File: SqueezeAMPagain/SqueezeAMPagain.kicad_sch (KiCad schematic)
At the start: 6 parts

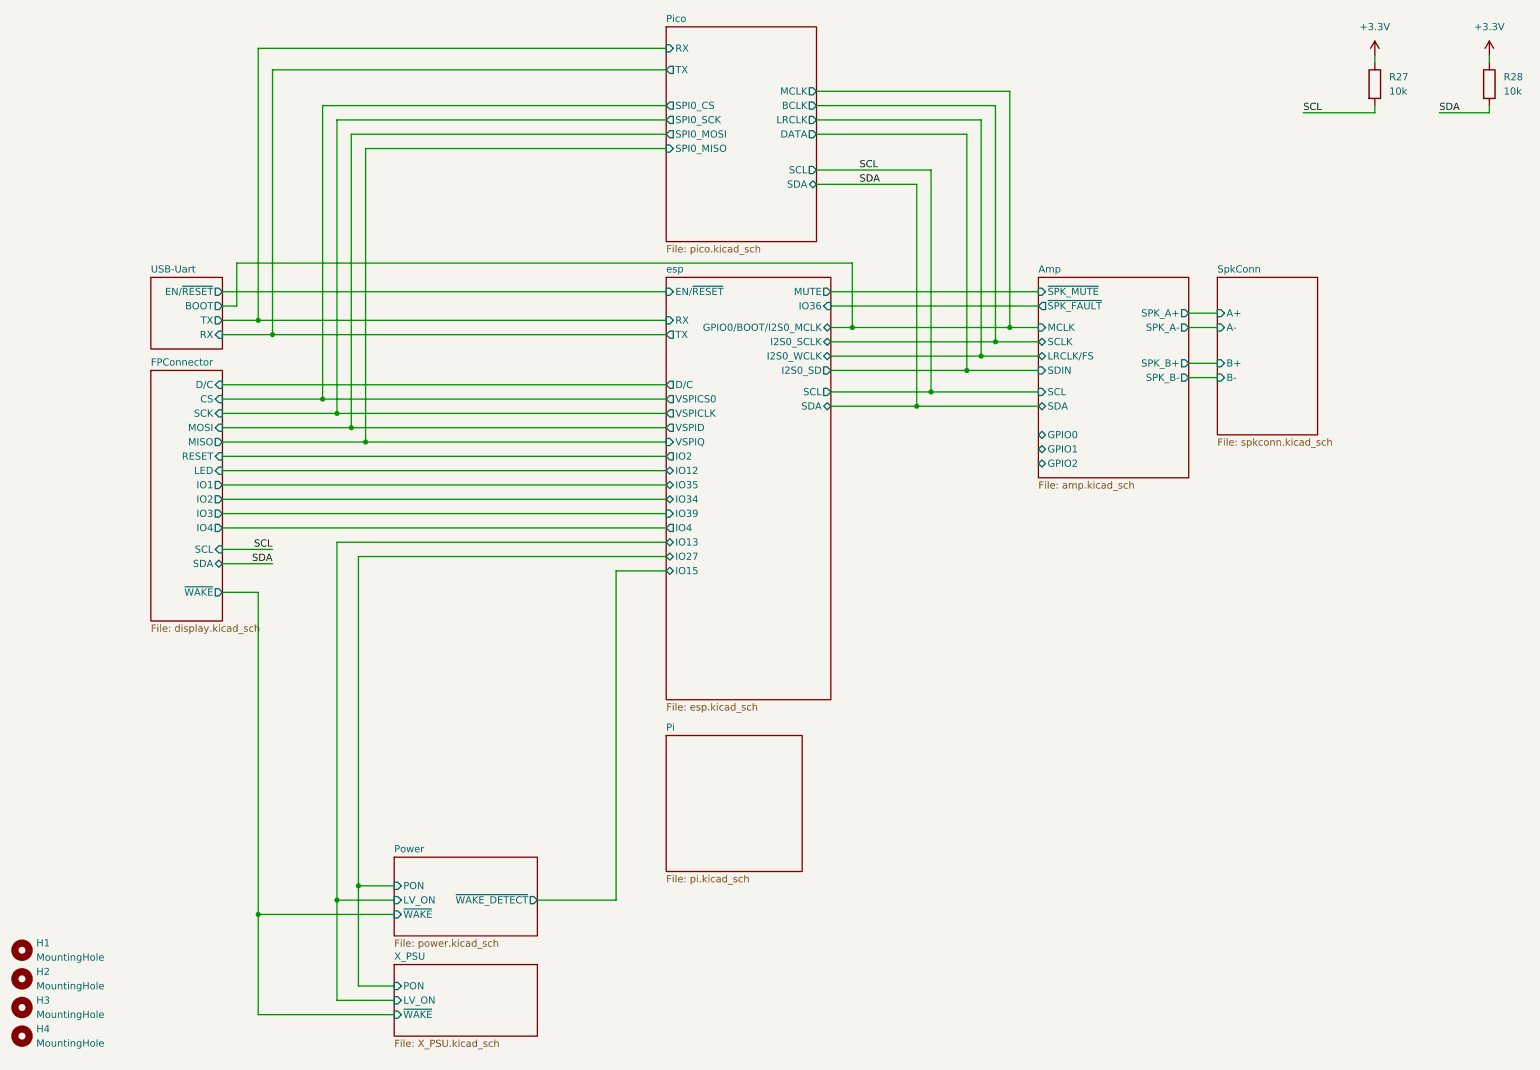
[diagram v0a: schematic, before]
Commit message: Update SqueezeAMPagain.kicad_pcb, SqueezeAMPagain.kicad_prl, SqueezeAMPagain.kicad_pro, and 7 more files
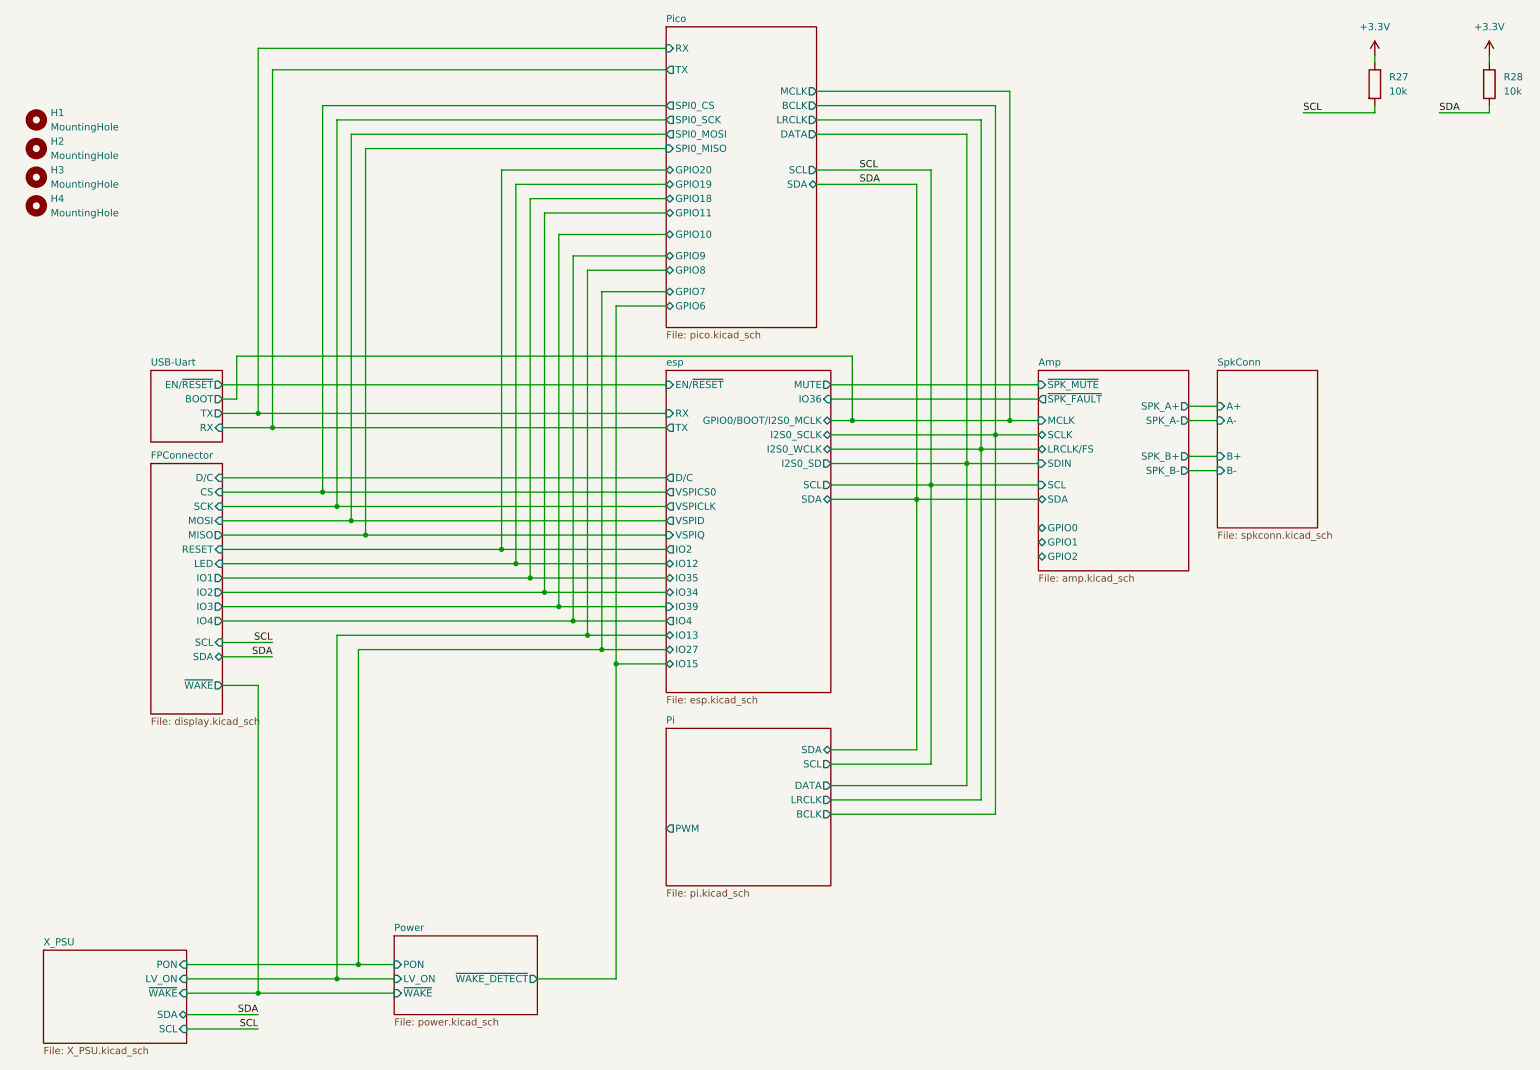
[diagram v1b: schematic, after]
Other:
- sheet Pi ports: added BCLK, DATA, LRCLK, PWM, SCL, SDA; removed none
- sheet Pico ports: added GPIO10, GPIO11, GPIO18, GPIO19, GPIO20, GPIO6, GPIO7, GPIO8, GPIO9; removed none
- sheet X_PSU ports: added SCL, SDA; removed none
- moved on the sheet: H1, H2, H3, H4

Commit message: Update L_Radial_D12.0mm_P5+6+7.00mm_Fastron_11P.kicad_mod, SqueezeAMPagain.kicad_pcb, SqueezeAMPagain.kicad_prl, and 5 more files
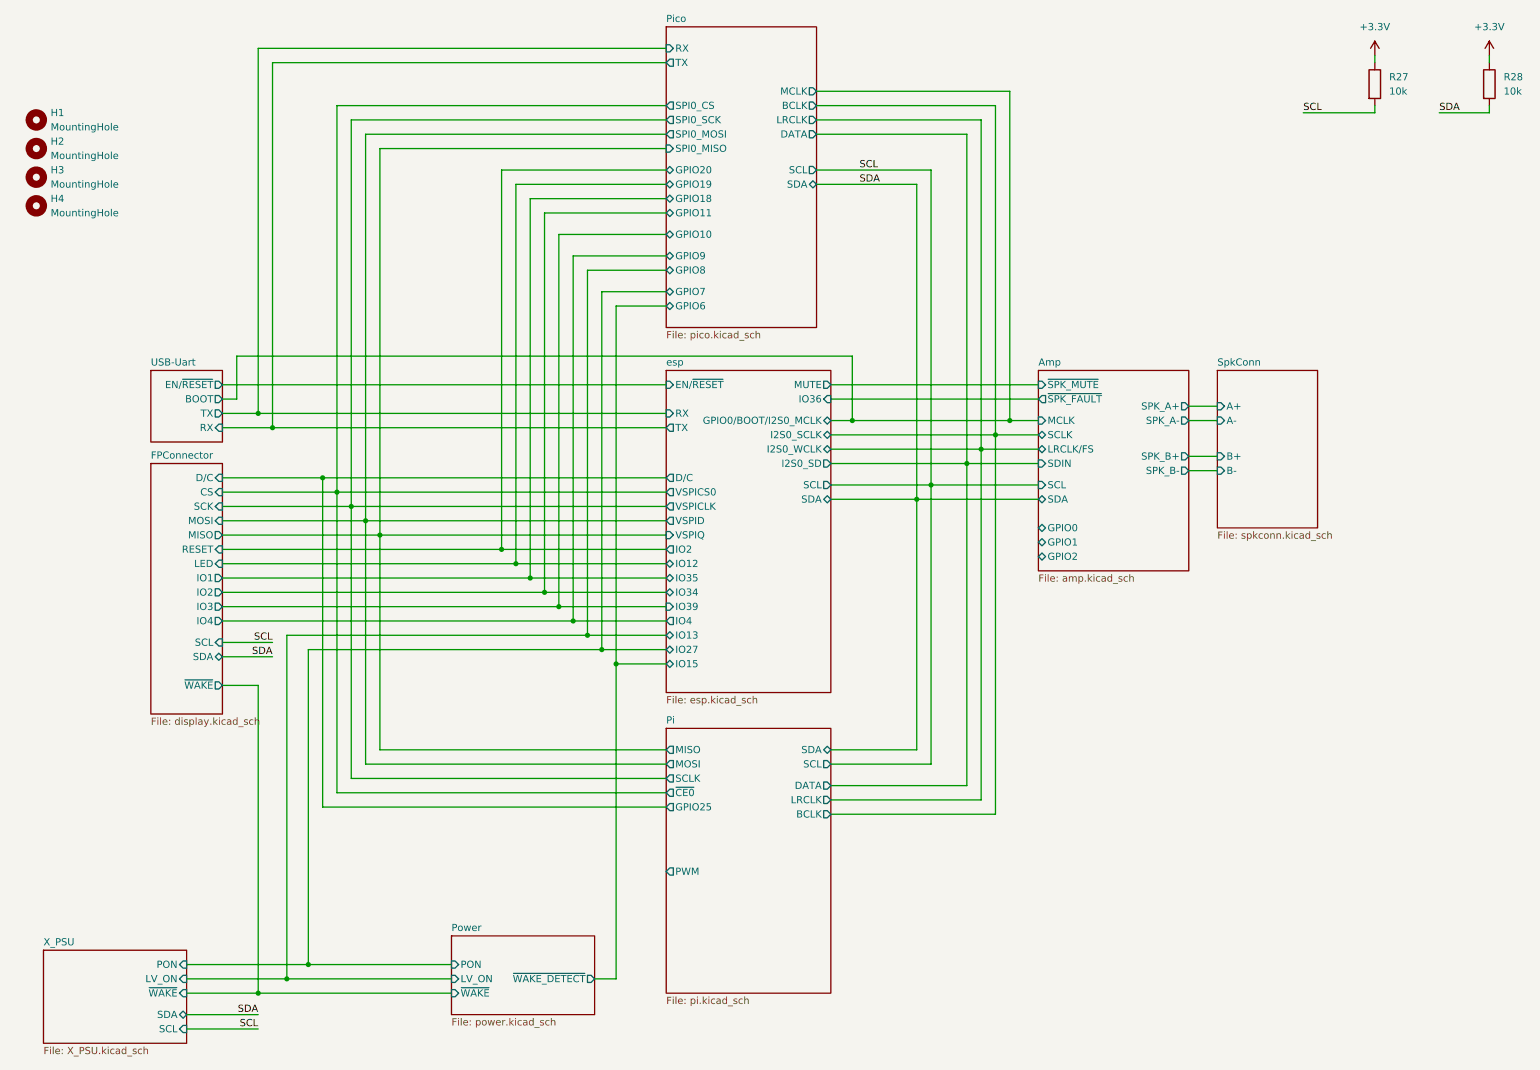
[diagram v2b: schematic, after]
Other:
- sheet Pi ports: added GPIO25, MISO, MOSI, SCLK, ~{CE0}; removed none
